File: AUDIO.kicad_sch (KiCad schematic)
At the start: 16 parts, among them J6 SJ-3524-SMT, U7 TLV320AIC3100

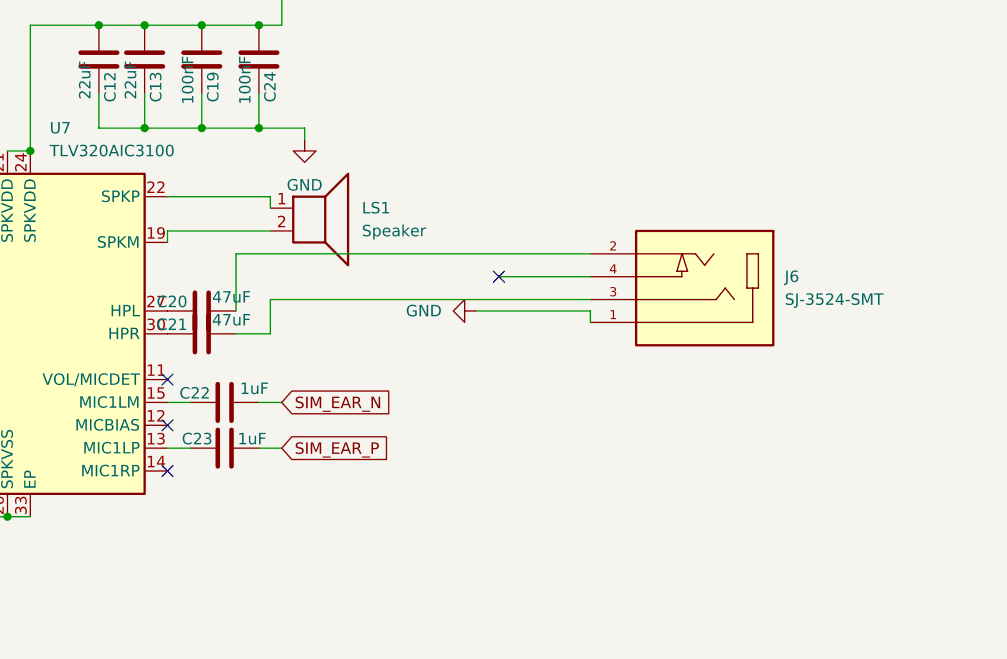
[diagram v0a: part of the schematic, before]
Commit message: P
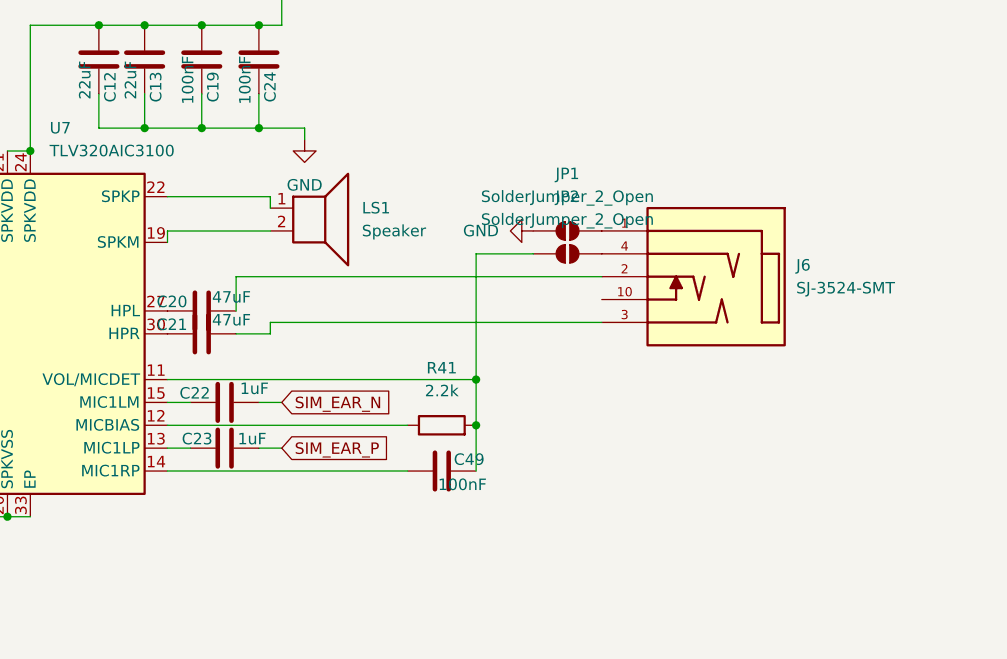
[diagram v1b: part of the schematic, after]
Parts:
- added C49: 100nF, Capacitor_SMD:C_0603_1608Metric_Pad1.08x0.95mm_HandSolder, symbol Device:C
- added JP1, JP2: SolderJumper_2_Open, Jumper:SolderJumper-2_P1.3mm_Open_TrianglePad1.0x1.5mm, symbol Jumper:SolderJumper_2_Open
- added R41: 2.2k, symbol Device:R
- J6: footprint Connector_Audio:Jack_3.5mm_CUI_SJ-3524-SMT_Horizontal -> 35RASMT6CHNTRX:SWITCHCRAFT_35RASMT6CHNTRX; symbol SJ-3524-SMT:SJ-3524-SMT -> 35RASMT6CHNTRX:35RASMT6CHNTRX; MANUFACTURER (none) -> Switchcraft; MAXIMUM_PACKAGE_HEIGHT (none) -> 5.1mm; PARTREV 1.03 -> A; STANDARD Manufacturer recommendations -> Manufacturer Recommendations
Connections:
- net GND: now also JP1.1 (A); no longer J6.1
- net at J6.4: now also JP2.2 (B)
- net at U7.11 (VOL/MICDET): now also C49.1, JP2.1 (A), R41.2
- net at U7.12 (MICBIAS): now also R41.1
- net at U7.14 (MIC1RP): now also C49.2
- new net: J6.1, JP1.2 (B)
- no-connect marks 4 -> 0
